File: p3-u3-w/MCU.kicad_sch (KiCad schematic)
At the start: 32 parts, among them J1 SWD_pin, J8 CONMHF1-SMD-G-T, SW2 SW_SPST, U3 STM32WB55CEUx, U7 DLF162500LT-5028A1, X1 NX2016SA-32MHZ-EXS00A-CS06654, Y2 32k768

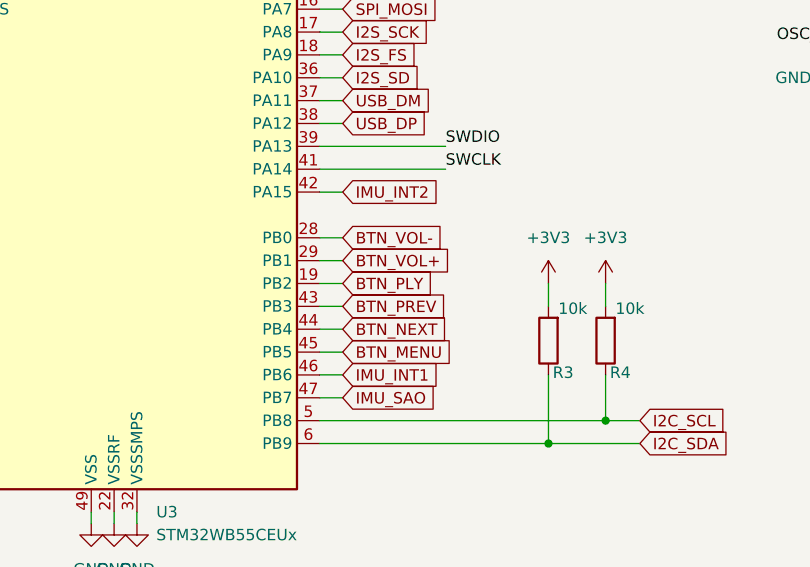
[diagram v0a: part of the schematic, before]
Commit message: did some more routing.
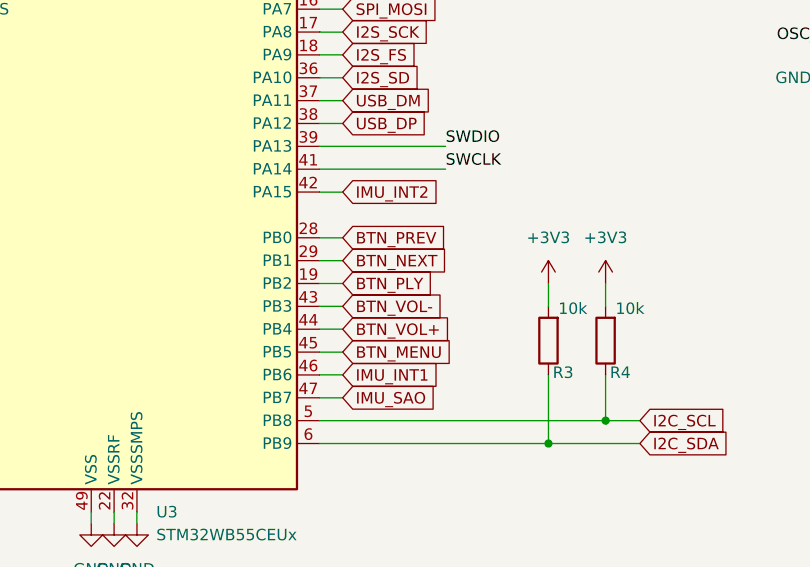
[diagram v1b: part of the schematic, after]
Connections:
- net BTN_NEXT: now also U3.29 (PB1); no longer U3.44 (PB4)
- net BTN_PREV: now also U3.28 (PB0); no longer U3.43 (PB3)
- net BTN_VOL+: now also U3.44 (PB4); no longer U3.29 (PB1)
- net BTN_VOL-: now also U3.43 (PB3); no longer U3.28 (PB0)

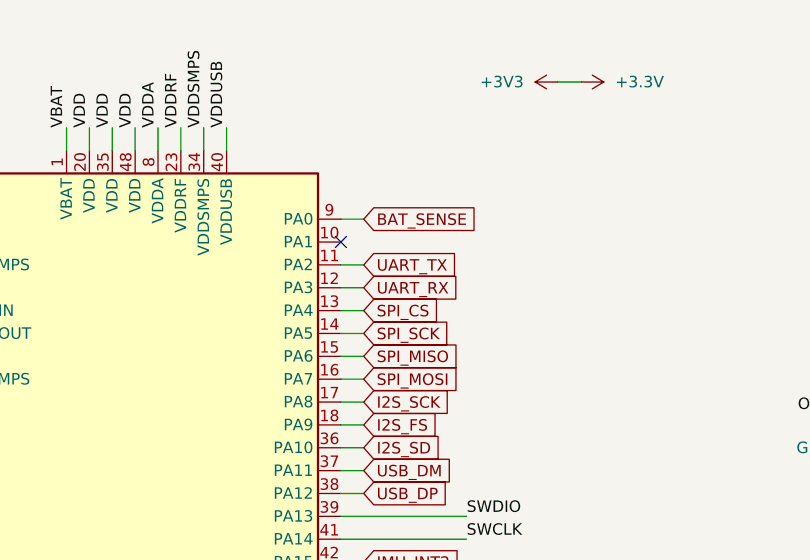
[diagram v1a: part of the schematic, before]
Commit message: finished the pcb, added in BOM
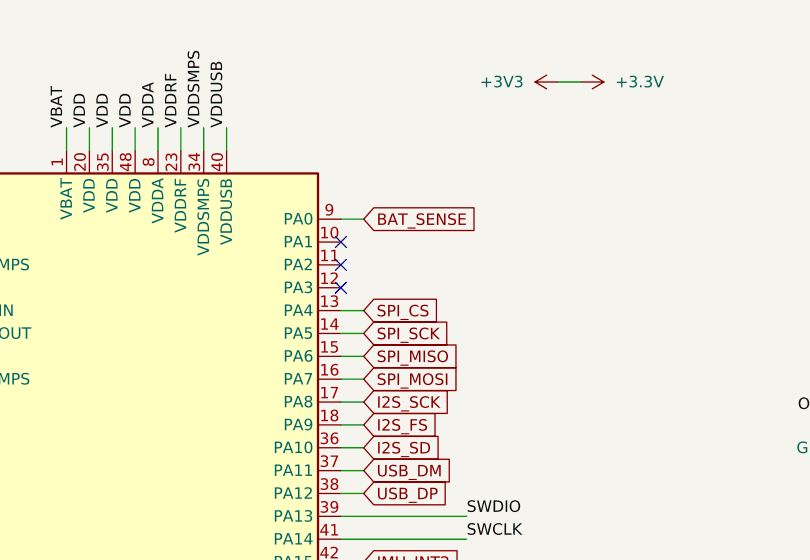
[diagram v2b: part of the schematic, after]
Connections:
- net UART_RX: no longer names the net of U3.12 (PA3)
- net UART_TX: no longer names the net of U3.11 (PA2)
- no-connect marks 2 -> 4
